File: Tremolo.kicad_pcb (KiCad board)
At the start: 2 copper layers, 177.9 x 90.1 mm, 113 parts, among them J1 Input, J10 R1, J11 R2, J12 TRG, J13 GND, J1A1 LeftA, J1B1 LeftB, J1C1 LeftC, J2 GND, J2A1 SwitchA, J2B1 SwitchB, J2C1 SwitchC, J3 +9v, J3A1 RightA, J3B1 RightB, J3C1 RightC, J4 GND, J5 RateSlv, J6 Gnd, J7 L2, J8 L1, J9 RateTip, Q1 BC549C, Q2 BC549C, Q3 BC549C, Q4 J113, Q5 BC549C, Q6 BC549C, T1 LeftTr, T2 RightTr, U1 TL072, U2 TL072, U3 TL072, U4 TL074, U5 VACTL, U6 VACTR

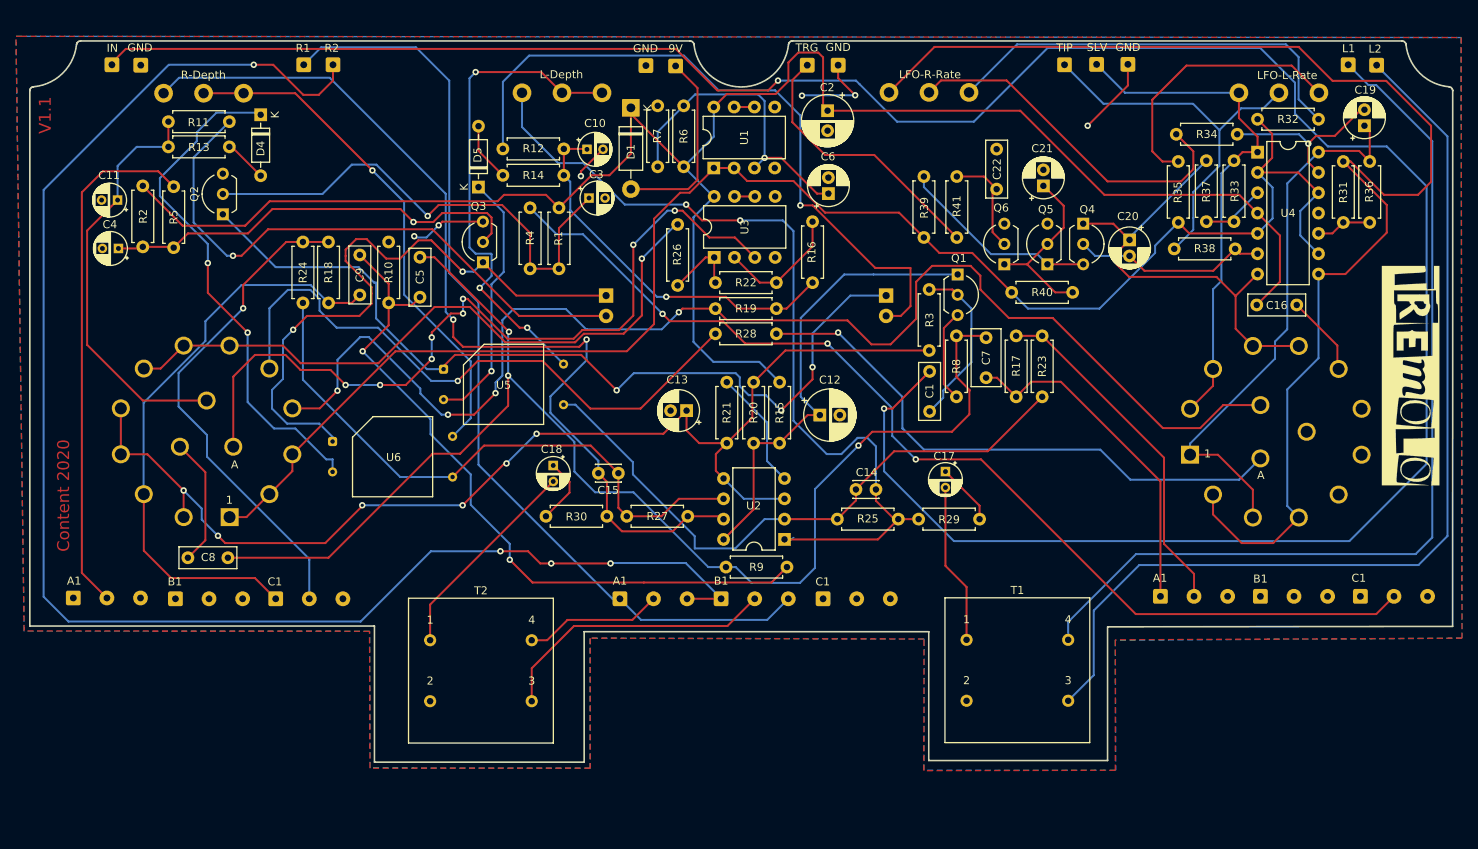
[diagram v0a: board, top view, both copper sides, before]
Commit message: V2.0 provisionaly completed
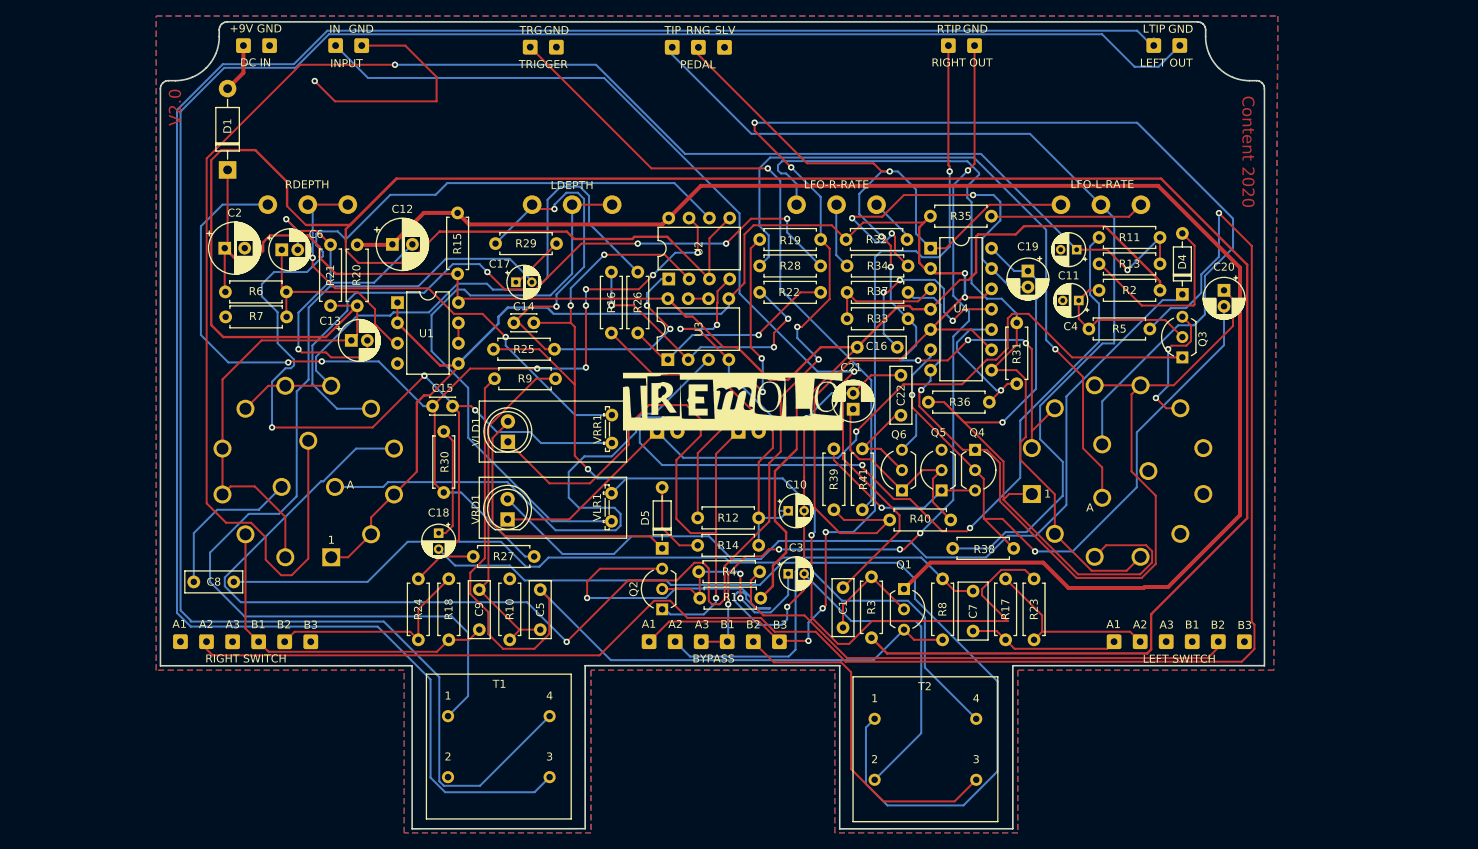
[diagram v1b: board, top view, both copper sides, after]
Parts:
- removed D2, D3: LED, LED_THT:LED_D5.0mm
- removed J1A1: LeftA, Connector_Wire:SolderWire-0.25sqmm_1x03_P4.2mm_D0.65mm_OD1.7mm
- removed J1B1: LeftB, Connector_Wire:SolderWire-0.25sqmm_1x03_P4.2mm_D0.65mm_OD1.7mm
- removed J1C1: LeftC, Connector_Wire:SolderWire-0.25sqmm_1x03_P4.2mm_D0.65mm_OD1.7mm
- removed J2A1: SwitchA, Connector_Wire:SolderWire-0.25sqmm_1x03_P4.2mm_D0.65mm_OD1.7mm
- removed J2B1: SwitchB, Connector_Wire:SolderWire-0.25sqmm_1x03_P4.2mm_D0.65mm_OD1.7mm
- removed J2C1: SwitchC, Connector_Wire:SolderWire-0.25sqmm_1x03_P4.2mm_D0.65mm_OD1.7mm
- removed J3A1: RightA, Connector_Wire:SolderWire-0.25sqmm_1x03_P4.2mm_D0.65mm_OD1.7mm
- removed J3B1: RightB, Connector_Wire:SolderWire-0.25sqmm_1x03_P4.2mm_D0.65mm_OD1.7mm
- removed J3C1: RightC, Connector_Wire:SolderWire-0.25sqmm_1x03_P4.2mm_D0.65mm_OD1.7mm
- removed U5: VACTL, OptoDevice:PerkinElmer_VTL5C
- removed U6: VACTR, OptoDevice:PerkinElmer_VTL5C
- added DL3: LED, LED_THT:LED_D5.0mm, B.Cu at (135.3, 89.5)
- added DR2: LED, LED_THT:LED_D5.0mm, B.Cu at (125.1, 89.5)
- added J14: LSB1, Connector_Wire:SolderWire-0.25sqmm_1x01_D0.65mm_OD1.7mm, F.Cu at (192.0, 115.8)
- added J15: RSA1, Connector_Wire:SolderWire-0.25sqmm_1x01_D0.65mm_OD1.7mm, F.Cu at (65.5, 115.8)
- added J16: LSB2, Connector_Wire:SolderWire-0.25sqmm_1x01_D0.65mm_OD1.7mm, F.Cu at (195.2, 115.8)
- added J17: RSA2, Connector_Wire:SolderWire-0.25sqmm_1x01_D0.65mm_OD1.7mm, F.Cu at (68.8, 115.8)
- added J18: RSA3, Connector_Wire:SolderWire-0.25sqmm_1x01_D0.65mm_OD1.7mm, F.Cu at (72.0, 115.8)
- added J19: LSB3, Connector_Wire:SolderWire-0.25sqmm_1x01_D0.65mm_OD1.7mm, F.Cu at (198.5, 115.8)
- added J20: LSA1, Connector_Wire:SolderWire-0.25sqmm_1x01_D0.65mm_OD1.7mm, F.Cu at (182.2, 115.8)
- added J21: RSB1, Connector_Wire:SolderWire-0.25sqmm_1x01_D0.65mm_OD1.7mm, F.Cu at (75.3, 115.8)
- added J22: LSA3, Connector_Wire:SolderWire-0.25sqmm_1x01_D0.65mm_OD1.7mm, F.Cu at (188.7, 115.8)
- added J23: RSB3, Connector_Wire:SolderWire-0.25sqmm_1x01_D0.65mm_OD1.7mm, F.Cu at (81.8, 115.8)
- added J24: LSA2, Connector_Wire:SolderWire-0.25sqmm_1x01_D0.65mm_OD1.7mm, F.Cu at (185.5, 115.8)
- added J25: RSB2, Connector_Wire:SolderWire-0.25sqmm_1x01_D0.65mm_OD1.7mm, F.Cu at (78.5, 115.8)
- added J26: SWA1, Connector_Wire:SolderWire-0.25sqmm_1x01_D0.65mm_OD1.7mm, F.Cu at (124.1, 115.8)
- added J27: SWA2, Connector_Wire:SolderWire-0.25sqmm_1x01_D0.65mm_OD1.7mm, F.Cu at (127.4, 115.8)
- added J28: SWA3, Connector_Wire:SolderWire-0.25sqmm_1x01_D0.65mm_OD1.7mm, F.Cu at (130.6, 115.8)
- added J29: SWB1, Connector_Wire:SolderWire-0.25sqmm_1x01_D0.65mm_OD1.7mm, F.Cu at (133.9, 115.8)
- added J30: SWB2, Connector_Wire:SolderWire-0.25sqmm_1x01_D0.65mm_OD1.7mm, F.Cu at (137.1, 115.8)
- added J31: SWB3, Connector_Wire:SolderWire-0.25sqmm_1x01_D0.65mm_OD1.7mm, F.Cu at (140.4, 115.8)
- added VLD1: D_Photo, MyLibrary:LED_D5.0mm, F.Cu at (106.4, 90.8)
- added VLR1: D_LDR, MyLibrary:R_LDR_5.2x5.2mm_P3.5mm_Horizontal, F.Cu at (119.4, 100.8)
- added VRD1: D_Photo, MyLibrary:LED_D5.0mm, F.Cu at (106.4, 100.5)
- added VRR1: D_LDR, MyLibrary:R_LDR_5.2x5.2mm_P3.5mm_Horizontal, F.Cu at (119.4, 91.0)
- Q1, Q2, Q3, Q4, Q5, Q6: footprint Package_TO_SOT_THT:TO-92L_Inline_Wide -> MyLibrary:TO-92L_Inline_Wide
- moved C4 120.2 mm to (177.8, 73.2)
- moved C11 120.0 mm to (177.5, 66.8)
- moved R2 119.7 mm to (180.3, 71.9), turned to 0 degrees
- moved D4 117.4 mm to (190.8, 72.4), turned to 90 degrees
- moved R5 114.9 mm to (179.1, 76.7), turned to 0 degrees
- moved R13 109.7 mm to (180.3, 68.6), turned to 0 degrees
- moved R11 109.7 mm to (180.3, 65.3), turned to 0 degrees
- moved Q3 88.2 mm to (190.8, 80.3)
- moved G*** 84.8 mm to (134.5, 85.8), turned to 0 degrees
- moved J10 80.6 mm to (161.5, 41.3)
- moved J11 80.2 mm to (164.8, 41.3)
- moved C2 77.3 mm to (71.0, 66.6), turned to 0 degrees
- moved Q2 73.8 mm to (125.7, 111.8)
- moved C6 68.7 mm to (78.2, 66.8), turned to 0 degrees
- moved T1 65.5 mm to (111.7, 125.1)
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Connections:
- net /LB1 renamed Net-(C14-Pad2)
- net /RB1 renamed Net-(C15-Pad2)
- C7 pad 2: Net-(C5-Pad2) -> Net-(C7-Pad2)
- C8 pad 2: Net-(C5-Pad2) -> Net-(C7-Pad2)
- D4 pad 1: /RA1 -> Net-(D4-Pad1)
- D5 pad 1: /LA1 -> Net-(D5-Pad1)
- Q1 pad 3: Net-(Q1-Pad3) -> Net-(C5-Pad2)
- Q2 pad 1: /LA2 -> Net-(DL3-Pad1)
- Q3 pad 1: /RA2 -> Net-(DR2-Pad1)
- R8 pad 1: Net-(Q1-Pad3) -> Net-(C5-Pad2)
- R8 pad 2: Net-(C5-Pad2) -> Net-(C7-Pad2)
- RV1 pad 1: /LB2 -> Net-(C14-Pad1)
- RV1 pad 2: /LB2 -> Net-(RV1-Pad2)
- RV1 pad 3: Net-(C14-Pad1) -> Net-(RV1-Pad2)
- RV2 pad 1: /RB2 -> Net-(C15-Pad1)
- RV2 pad 2: /RB2 -> Net-(RV2-Pad2)
- RV2 pad 3: Net-(C15-Pad1) -> Net-(RV2-Pad2)
- RV3 pad 1: Net-(R32-Pad2) -> /Shape4
- RV3 pad 3: /Shape4 -> Net-(R32-Pad2)
- RV4 pad 1: Net-(R35-Pad2) -> /Shape12
- RV4 pad 3: /Shape12 -> Net-(R35-Pad2)
- U1 pad 5: GND -> VDC
- U3 pad 5: GND -> VDC
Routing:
- net VAA: track 146.9 -> 398.6 mm, vias 6 -> 0
- net GND: track 60.2 -> 291.2 mm, vias 6 -> 13
- net Net-(C1-Pad2): track 308.9 -> 121.0 mm, vias 2 -> 1
- net /MODEB: track 52.2 -> 216.4 mm, vias 0 -> 2
- net Net-(J17-Pad1): track 65.4 -> 214.4 mm, vias 0 -> 1
- net Net-(J7-Pad1): track 116.1 -> 260.6 mm
- net +9VA: track 58.4 -> 198.2 mm
- net Net-(J8-Pad1): track 123.2 -> 254.6 mm
- net Net-(D4-Pad1): track 0.00 -> 112.7 mm
- net /MODE4: track 163.1 -> 275.5 mm, vias 4 -> 5
- net /LA2: track 109.1 -> 0.00 mm, vias 3 -> 0
- net Net-(DR2-Pad1): track 0.00 -> 102.7 mm, vias 0 -> 1
- net Net-(C17-Pad2): track 20.1 -> 119.7 mm
- net Net-(C7-Pad2): track 0.00 -> 98.5 mm
- net Net-(C18-Pad2): track 26.2 -> 119.6 mm
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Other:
- board size 177.9 x 90.1 mm -> 138 x 100.9 mm
- net class Power added: clearance 0.5, trace_width 0.5, via_dia 0.8, via_drill 0.4
- net class Power2 added: clearance 0.3, trace_width 0.3, via_dia 0.8, via_drill 0.4
- board text added: "+9V"
- board text added: "A2"
- board text added: "A3"
- board text added: "B2"
- board text added: "B3"
- board text added: "BYPASS"
- board text added: "DC IN"
- board text added: "INPUT"
- board text added: "LDEPTH"
- board text added: "LEFT OUT"
- board text added: "LEFT SWITCH"
- board text added: "LFO-L-RATE"
- board text added: "LFO-R-RATE"
- board text added: "LTIP"
- board text added: "PEDAL"
- board text added: "RDEPTH"
- board text added: "RIGHT OUT"
- board text added: "RIGHT SWITCH"
- board text added: "RNG"
- board text added: "RTIP"
- board text added: "TRIGGER"
- board text added: "V2.0"
- board text removed: "9V"
- board text removed: "C1"
- board text removed: "L-Depth"
- board text removed: "L1"
- board text removed: "L2"
- board text removed: "LFO-L-Rate"
- board text removed: "LFO-R-Rate"
- board text removed: "R-Depth"
- board text removed: "R1"
- board text removed: "R2"
- board text removed: "V1.1"
